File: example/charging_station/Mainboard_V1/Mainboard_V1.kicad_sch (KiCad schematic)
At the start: 33 parts, among them J1 Screw_Terminal_01x02, J2 Conn_01x04_Pin, J3 Conn_01x04_Socket, J4 Conn_01x04_Pin, J6 Conn_02x04_Counter_Clockwise, J7 Conn_02x04_Counter_Clockwise, J8 Conn_02x04_Counter_Clockwise, U1 DRV8834

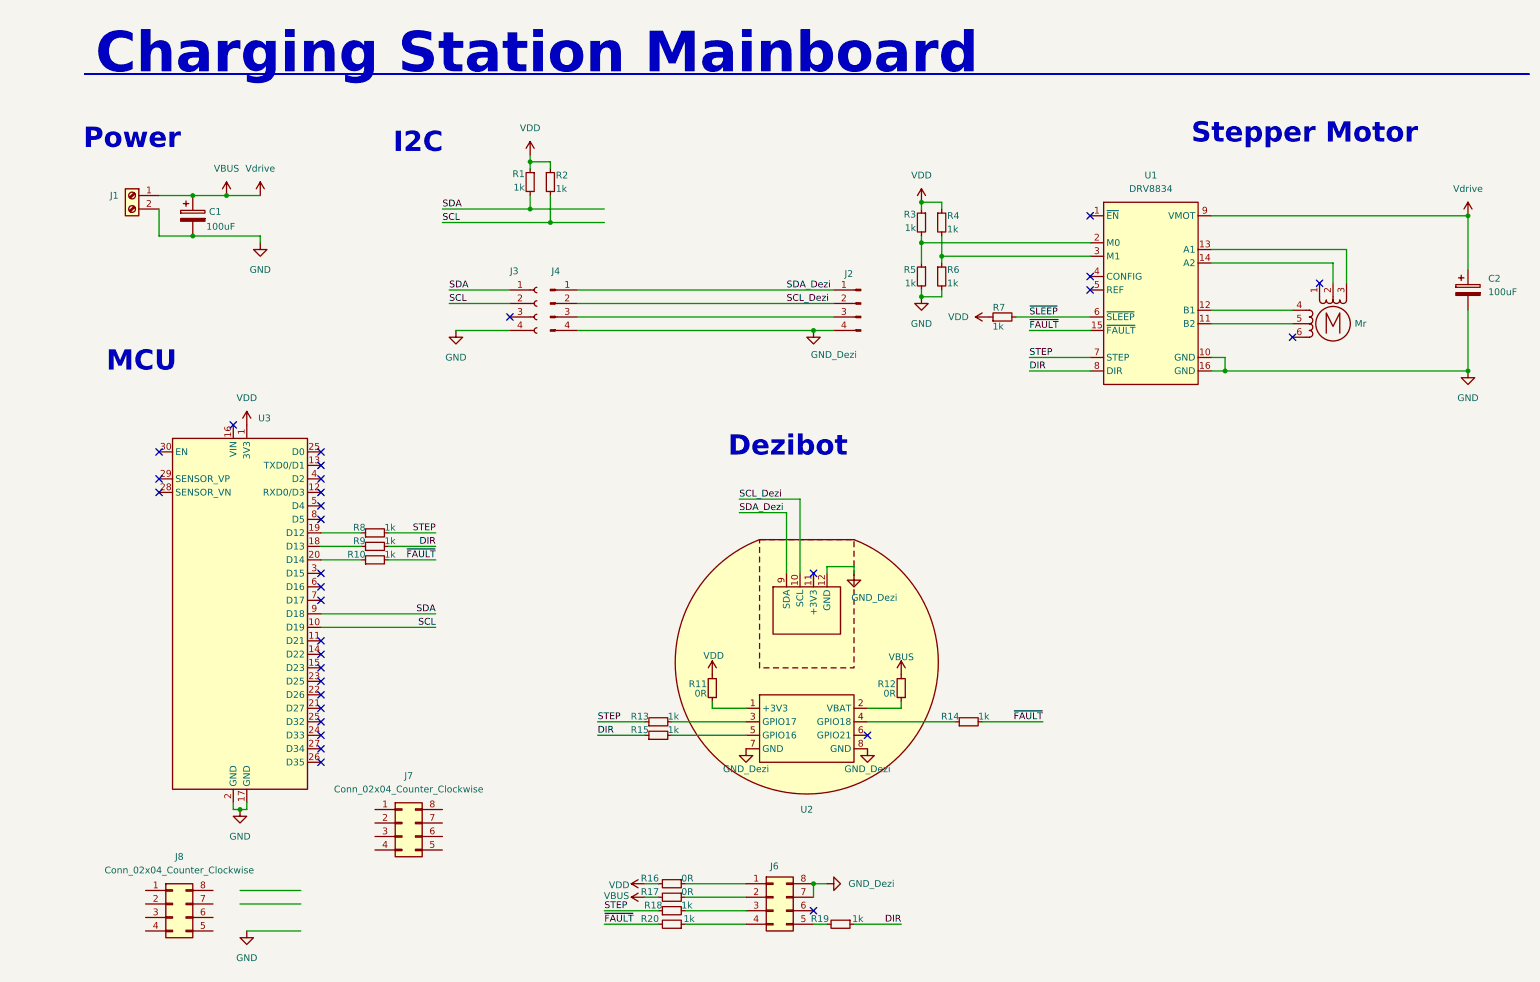
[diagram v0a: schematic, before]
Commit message: Update PCB
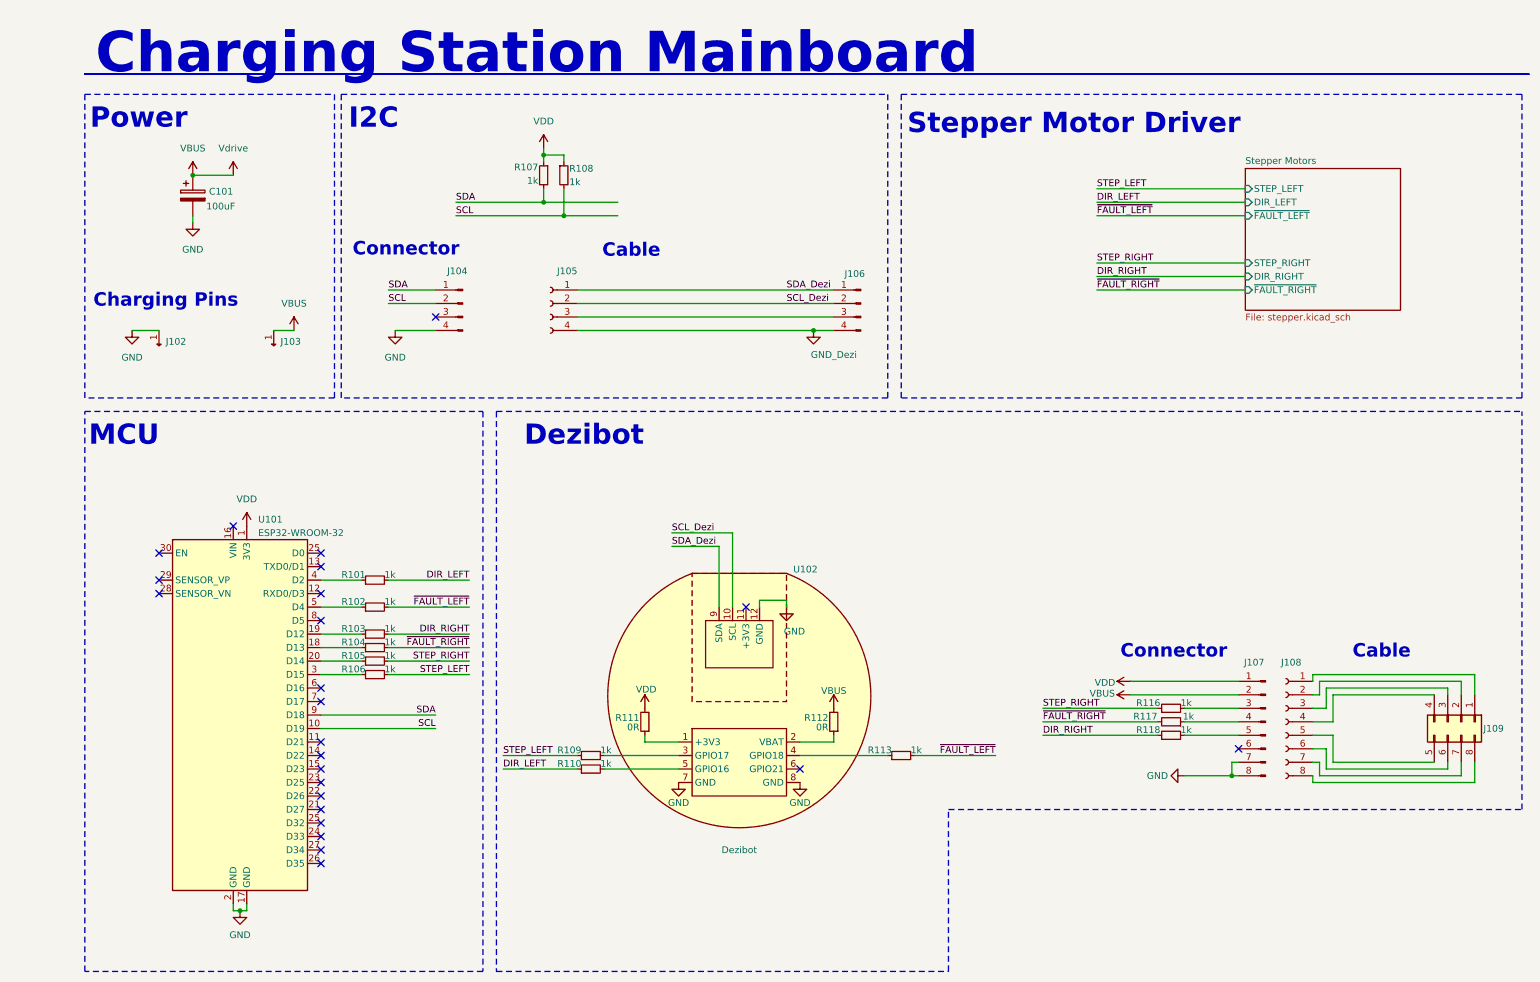
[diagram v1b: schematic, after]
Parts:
- removed C2: 100uF, Capacitor_THT:CP_Radial_D4.0mm_P1.50mm, symbol Device:C_Polarized
- removed J1: Screw_Terminal_01x02, symbol Connector:Screw_Terminal_01x02
- removed J7, J8: Conn_02x04_Counter_Clockwise, symbol Connector_Generic:Conn_02x04_Counter_Clockwise
- removed Mr: Stepper_Motor_unipolar_6pin, symbol Motor:Stepper_Motor_unipolar_6pin
- removed R16, R17: 0R, symbol Device:R_Small
- removed R3, R4, R5, R6, R7: 1k, symbol Device:R_Small
- removed U1: DRV8834, Mainboard:Polulu_DRV8834, symbol Mainboard:Polulu_DRV8834
- added J102, J103: ~, Mainboard:PogoPin, symbol Mainboard:PogoPin
- added J107: Conn_01x08_Pin, Connector_PinHeader_2.54mm:PinHeader_1x08_P2.54mm_Vertical, symbol Connector:Conn_01x08_Pin
- added J108: Conn_01x08_Socket, symbol Connector:Conn_01x08_Socket
- added R101, R102, R106: 1k, Resistor_THT:R_Axial_DIN0207_L6.3mm_D2.5mm_P10.16mm_Horizontal, symbol Device:R_Small
- J104: renamed from J4; footprint (none) -> Connector_PinHeader_2.54mm:PinHeader_1x04_P2.54mm_Vertical
- R103: renamed from R8; footprint (none) -> Resistor_THT:R_Axial_DIN0207_L6.3mm_D2.5mm_P10.16mm_Horizontal
- R104: renamed from R9; footprint (none) -> Resistor_THT:R_Axial_DIN0207_L6.3mm_D2.5mm_P10.16mm_Horizontal
- R105: renamed from R10; footprint (none) -> Resistor_THT:R_Axial_DIN0207_L6.3mm_D2.5mm_P10.16mm_Horizontal
- R107: renamed from R1; footprint (none) -> Resistor_THT:R_Axial_DIN0207_L6.3mm_D2.5mm_P10.16mm_Horizontal
- R108: renamed from R2; footprint (none) -> Resistor_THT:R_Axial_DIN0207_L6.3mm_D2.5mm_P10.16mm_Horizontal
- R109: renamed from R13; footprint (none) -> Resistor_THT:R_Axial_DIN0207_L6.3mm_D2.5mm_P10.16mm_Horizontal
- R110: renamed from R15; footprint (none) -> Resistor_THT:R_Axial_DIN0207_L6.3mm_D2.5mm_P10.16mm_Horizontal
- R111: renamed from R11; footprint (none) -> Jumper:SolderJumper-2_P1.3mm_Open_RoundedPad1.0x1.5mm
- R112: renamed from R12; footprint (none) -> Jumper:SolderJumper-2_P1.3mm_Open_RoundedPad1.0x1.5mm
- R113: renamed from R14; footprint (none) -> Resistor_THT:R_Axial_DIN0207_L6.3mm_D2.5mm_P10.16mm_Horizontal
- R116: renamed from R18; footprint (none) -> Resistor_THT:R_Axial_DIN0207_L6.3mm_D2.5mm_P10.16mm_Horizontal
- R117: renamed from R20; footprint (none) -> Resistor_THT:R_Axial_DIN0207_L6.3mm_D2.5mm_P10.16mm_Horizontal
- R118: renamed from R19; footprint (none) -> Resistor_THT:R_Axial_DIN0207_L6.3mm_D2.5mm_P10.16mm_Horizontal
- U101: renamed from U3; value ~ -> ESP32-WROOM-32
- U102: renamed from U2; value ~ -> Dezibot
- renumbered C1 to C101, J3 to J105, J2 to J106, J6 to J109
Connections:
- net GND: now also J104.4 (Pin_4), U102.12 (GND), U102.7 (GND), U102.8 (GND), J102.1, J107.7 (Pin_7), J107.8 (Pin_8); no longer J105.4 (Pin_4)
- net GND_Dezi: now also J105.4 (Pin_4); no longer J104.4 (Pin_4), J109.7 (Pin_7), J109.8 (Pin_8), U102.12 (GND), U102.7 (GND), U102.8 (GND)
- net SCL: now also J104.2 (Pin_2); no longer J105.2 (Pin_2)
- net SCL_Dezi: now also J105.2 (Pin_2); no longer J104.2 (Pin_2)
- net SDA: now also J104.1 (Pin_1); no longer J105.1 (Pin_1)
- net SDA_Dezi: now also J105.1 (Pin_1); no longer J104.1 (Pin_1)
- net VBUS: now also J103.1, J107.2 (Pin_2)
- net VDD: now also J107.1 (Pin_1)
- net at U101.3 (D15): now also R106.1
- net at U101.4 (D2): now also R101.1
- net at U101.5 (D4): now also R102.1
- net at R118.2: now also J107.5 (Pin_5); no longer J109.5 (Pin_5)
- net at J109.1 (Pin_1): now also J108.1 (Pin_1)
- net at J104.3 (Pin_3): no longer J106.3 (Pin_3)
- net at J105.3 (Pin_3): now also J106.3 (Pin_3)
- net at J109.2 (Pin_2): now also J108.2 (Pin_2)
- net at R116.2: now also J107.3 (Pin_3); no longer J109.3 (Pin_3)
- net at R117.1: now also J107.4 (Pin_4); no longer J109.4 (Pin_4)
- net at J109.6 (Pin_6): now also J108.6 (Pin_6)
- removed net DIR: R104.2, R110.1, R118.1
- removed net STEP: R103.2, R109.1, R116.1
- removed net ~{FAULT}: R105.2, R113.2, R117.2
- new net: J108.3 (Pin_3), J109.3 (Pin_3)
- new net: J108.4 (Pin_4), J109.4 (Pin_4)
- new net: J108.5 (Pin_5), J109.5 (Pin_5)
- new net: J108.7 (Pin_7), J109.7 (Pin_7)
- new net: J108.8 (Pin_8), J109.8 (Pin_8)
- new net DIR_LEFT: R101.2, R110.1
- new net DIR_RIGHT: R103.2, R118.1
- new net STEP_LEFT: R106.2, R109.1
- new net STEP_RIGHT: R105.2, R116.1
- new net ~{FAULT_LEFT}: R102.2, R113.2
- new net ~{FAULT_RIGHT}: R104.2, R117.2
- now unconnected: U101.15 (D23)
- no-connect marks 32 -> 24
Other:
- added sheet Stepper Motors (stepper.kicad_sch)
- note added: "Cable"
- note added: "Charging Pins"
- note added: "Connector"
- note added: "Stepper Motor Driver"
- note removed: "Stepper Motor"
- moved on the sheet: C101, J104, J105, J109, R103, R104, R105, R107, R108, R109, R110, R111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

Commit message: PCB updates
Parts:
- C101: footprint Capacitor_THT:CP_Radial_D4.0mm_P1.50mm -> Capacitor_THT:CP_Radial_D4.0mm_P2.00mm
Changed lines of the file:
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@@
 			)
 		)
-		(property "Footprint" "Capacitor_THT:CP_Radial_D4.0mm_P1.50mm"
+		(property "Footprint" "Capacitor_THT:CP_Radial_D4.0mm_P2.00mm"
 			(at 33.9852 52.07 0)
 			(effects
